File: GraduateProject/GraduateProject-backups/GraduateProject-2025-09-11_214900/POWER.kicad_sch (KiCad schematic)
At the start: 24 parts, among them IC1 PIC16C620A-04/SS, IC2 PIC16C620A-04/SS, Q4 MMBT2222A, SW1 SS12D10G3, U5 B0505S-1W, U7 B0505S-1W

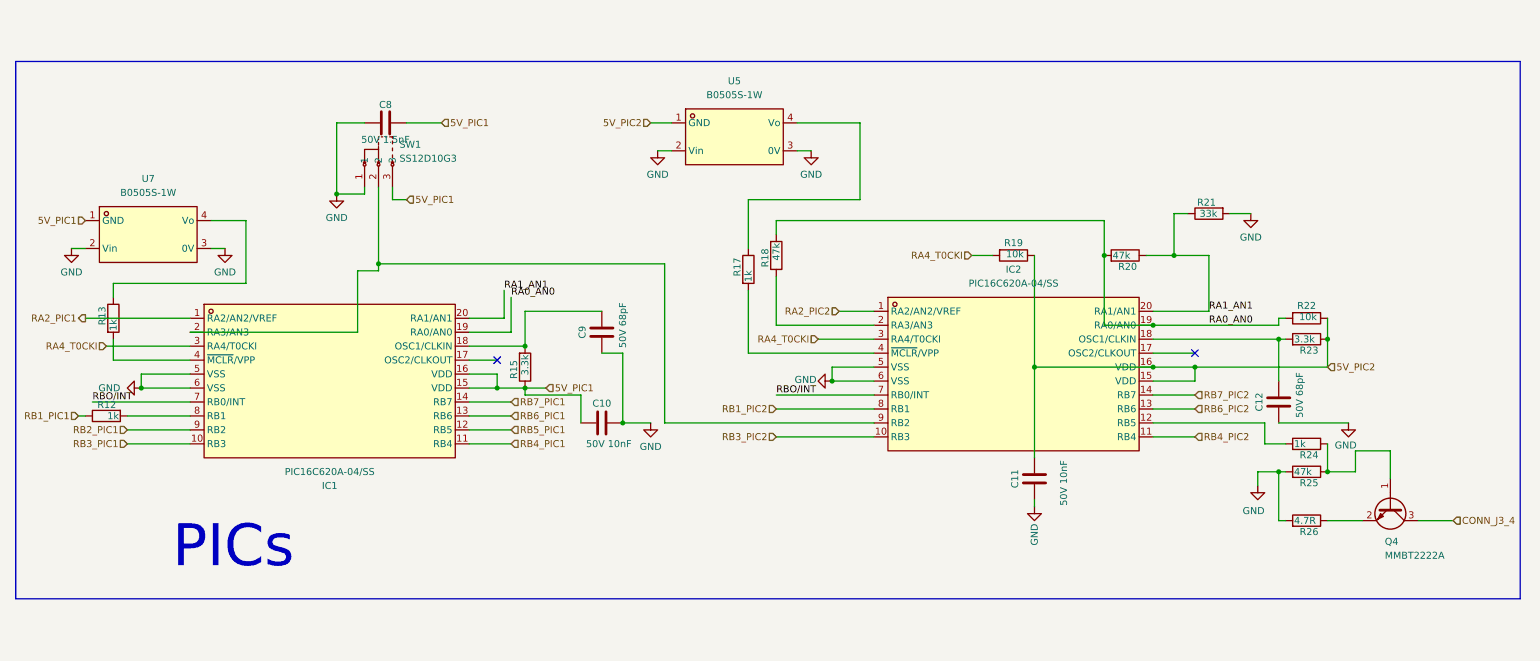
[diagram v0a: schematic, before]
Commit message: Add files via upload
18h02 12/9/25
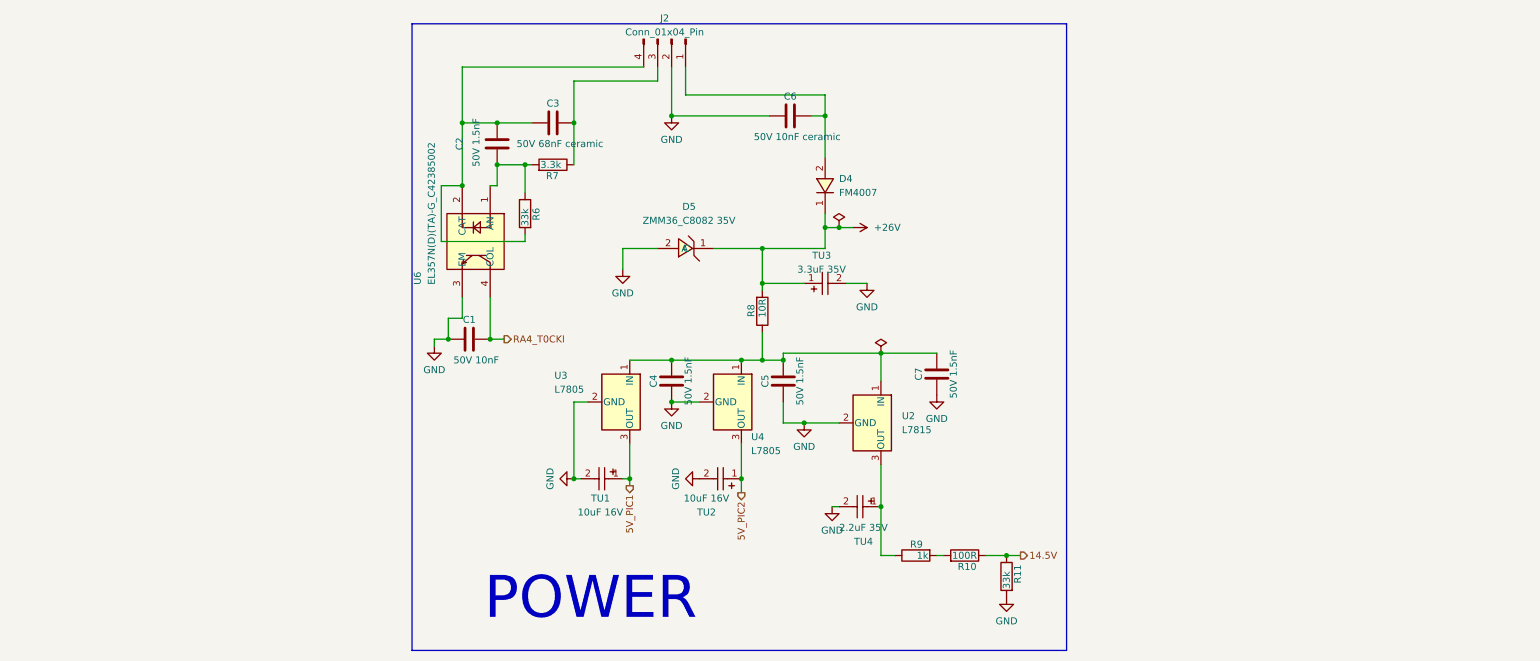
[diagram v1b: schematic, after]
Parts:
- removed C10, C11: 50V 10nF, Capacitor_SMD:C_0805_2012Metric, symbol Device:C
- removed C12, C9: 50V 68pF, Capacitor_SMD:C_0805_2012Metric, symbol Device:C
- removed C8: 50V 1.5nF, Capacitor_SMD:C_0805_2012Metric, symbol Device:C
- removed IC1, IC2: PIC16C620A-04/SS, easyeda2kicad:SSOP-20_L7.2-W5.3-P0.65-LS7.8-BL, symbol easyeda2kicad:PIC16C620A-04_SS
- removed Q4: MMBT2222A, Package_TO_SOT_SMD:SOT-23, symbol Transistor_BJT:MMBT2222A
- removed R12, R13, R17, R24: 1k, Resistor_SMD:R_0805_2012Metric, symbol Device:R
- removed R15, R23: 3.3k, Resistor_SMD:R_0805_2012Metric, symbol Device:R
- removed R18, R20, R25: 47k, Resistor_SMD:R_0805_2012Metric, symbol Device:R
- removed R19, R22: 10k, Resistor_SMD:R_0805_2012Metric, symbol Device:R
- removed R21: 33k, Resistor_SMD:R_0805_2012Metric, symbol Device:R
- removed R26: 4.7R, Resistor_SMD:R_0805_2012Metric, symbol Device:R
- removed SW1: SS12D10G3, easyeda2kicad:SW-TH_3P-P4.8-L12.7-W6.7_SS12D10G3, symbol easyeda2kicad:SS12D10G3
- removed U5, U7: B0505S-1W, easyeda2kicad:PWRM-TH_BXXXXS-1W, symbol easyeda2kicad:B0505S-1W
- added C1: 50V 10nF, Capacitor_SMD:C_0805_2012Metric, symbol Device:C
- added C2, C4, C5, C7: 50V 1.5nF, Capacitor_SMD:C_0805_2012Metric, symbol Device:C
- added C3: 50V 68nF ceramic, Capacitor_SMD:C_0805_2012Metric, symbol Device:C
- added C6: 50V 10nF ceramic, Capacitor_SMD:C_1206_3216Metric, symbol Device:C
- added D4: FM4007, easyeda2kicad:SOD-123FL_L2.7-W1.8-LS3.8-RD, symbol easyeda2kicad:FM4007
- added D5: ZMM36_C8082 35V, easyeda2kicad:LL-34_L3.5-W1.5-RD, symbol easyeda2kicad:ZMM33_C8082
- added J2: Conn_01x04_Pin, Connector_PinHeader_2.54mm:PinHeader_1x04_P2.54mm_Vertical, symbol Connector:Conn_01x04_Pin
- added R10: 100R, Resistor_SMD:R_0805_2012Metric, symbol Device:R
- added R11, R6: 33k, Resistor_SMD:R_0805_2012Metric, symbol Device:R
- added R7: 3.3k, Resistor_SMD:R_0805_2012Metric, symbol Device:R
- added R8: 10R, Resistor_SMD:R_0805_2012Metric, symbol Device:R
- added R9: 1k, Resistor_SMD:R_0805_2012Metric, symbol Device:R
- added TU1, TU2: 10uF 16V, easyeda2kicad:CAP-SMD_L3.2-W1.6-RD-C7171, symbol easyeda2kicad:TAJA106K016RNJ
- added TU3: 3.3uF 35V, easyeda2kicad:CAP-SMD_L3.5-W2.8-R-RD, symbol easyeda2kicad:TAJB335K035RNJ
- added TU4: 2.2uF 35V, easyeda2kicad:CAP-SMD_L3.5-W2.8-R-RD, symbol easyeda2kicad:TAJB225K035RNJ
- added U2: L7815, Package_TO_SOT_SMD:TO-263-2, symbol Regulator_Linear:L7815
- added U3, U4: L7805, Package_TO_SOT_SMD:TO-263-2, symbol Regulator_Linear:L7805
- added U6: EL357N(D)(TA)-G_C42385002, easyeda2kicad:SOP-4_L3.9-W4.4-P2.54-LS7.0-TL, symbol easyeda2kicad:EL357N(D)(TA)-G_C42385002
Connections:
- net 5V_PIC1: now also TU1.1, U3.3 (OUT)
- net 5V_PIC2: now also TU2.1, U4.3 (OUT)
- net GND: now also C1.2, C4.2, C5.2, C6.2, C7.2, D5.2 (A), J2.2 (Pin_2), R11.2, TU1.2, TU2.2, TU3.2, TU4.2, U2.2 (GND), U3.2 (GND), U4.2 (GND), U6.3 (EM)
- net RA4_T0CKI: now also C1.1, U6.4 (COL)
- new net: C2.2, R6.1, R7.2, U6.1 (AN)
- new net: C2.1, C3.2, J2.4 (Pin_4), R6.2, U6.2 (CAT)
- new net: R9.1, TU4.1, U2.3 (OUT)
- new net: R10.2, R9.2
- new net: C3.1, J2.3 (Pin_3), R7.1
- new net: C6.1, D4.2 (A), J2.1 (Pin_1)
- new net: C4.1, C5.1, C7.1, R8.1, U2.1 (IN), U3.1 (IN), U4.1 (IN)
- new net +26V: D4.1 (C), D5.1 (C), R8.2, TU3.1
- new net 14.5V: R10.1, R11.1
- no-connect marks 2 -> 0
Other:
- note added: "POWER"
- note removed: "PICs"
